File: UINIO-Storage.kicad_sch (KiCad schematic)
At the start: 36 parts, among them J1 Conn_01x04_Pin, J2 Conn_01x04_Pin, J3 Conn_01x06_Pin, J4 Conn_01x08_Pin, J5 Conn_01x06_Pin, U1 I2C-24-EEPROM-SOIC8, U2 I2C-24-EEPROM-TSSOP8, U3 SPI-25-Flash-SOIC8, U4 ME6211, U5 SPI-25-Flash-WSON8

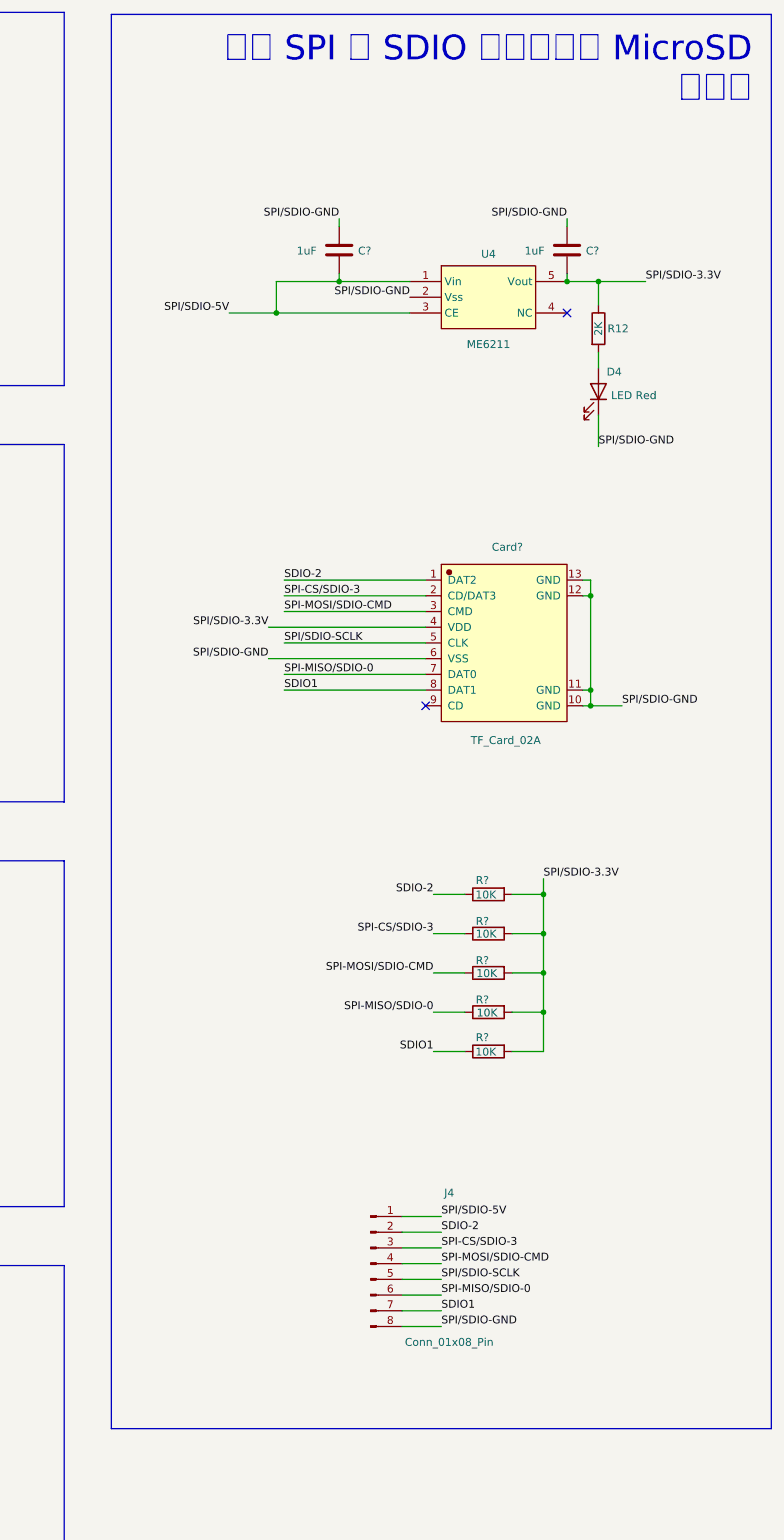
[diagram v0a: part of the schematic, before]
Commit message: Release UINIO-Storage version 1.0.0.
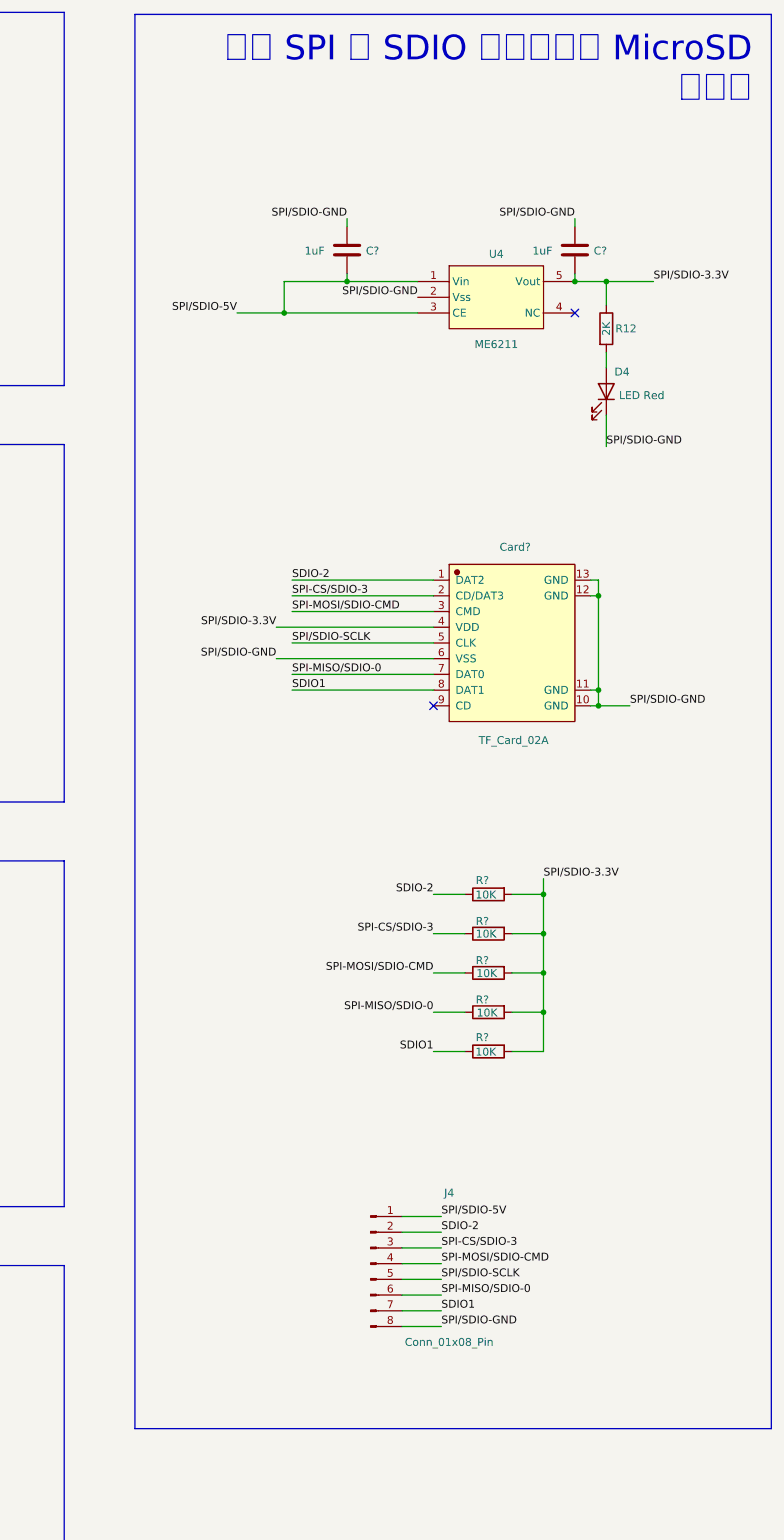
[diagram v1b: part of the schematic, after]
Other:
- company: 电子技术博客 UinIO.com -> UinIO.com 电子实验室
- moved on the sheet: C?, Card?, D4, R12, U4
